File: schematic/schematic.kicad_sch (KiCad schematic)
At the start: 7 parts, among them K1 TIANBO-HJR-4102-L, U1 Pico

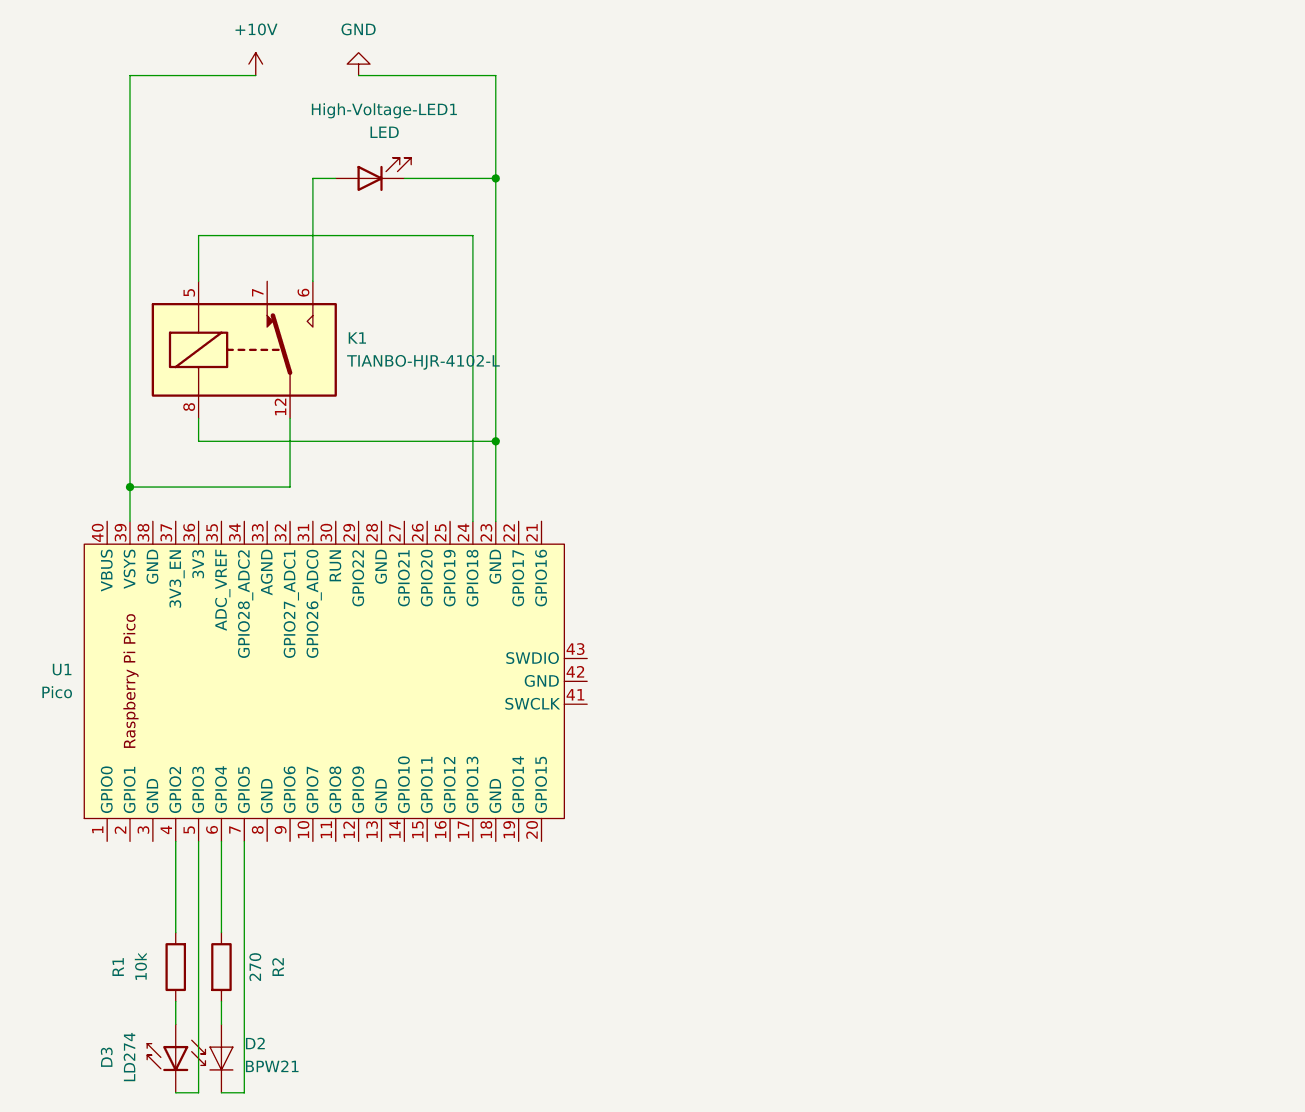
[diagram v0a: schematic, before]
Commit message: wip
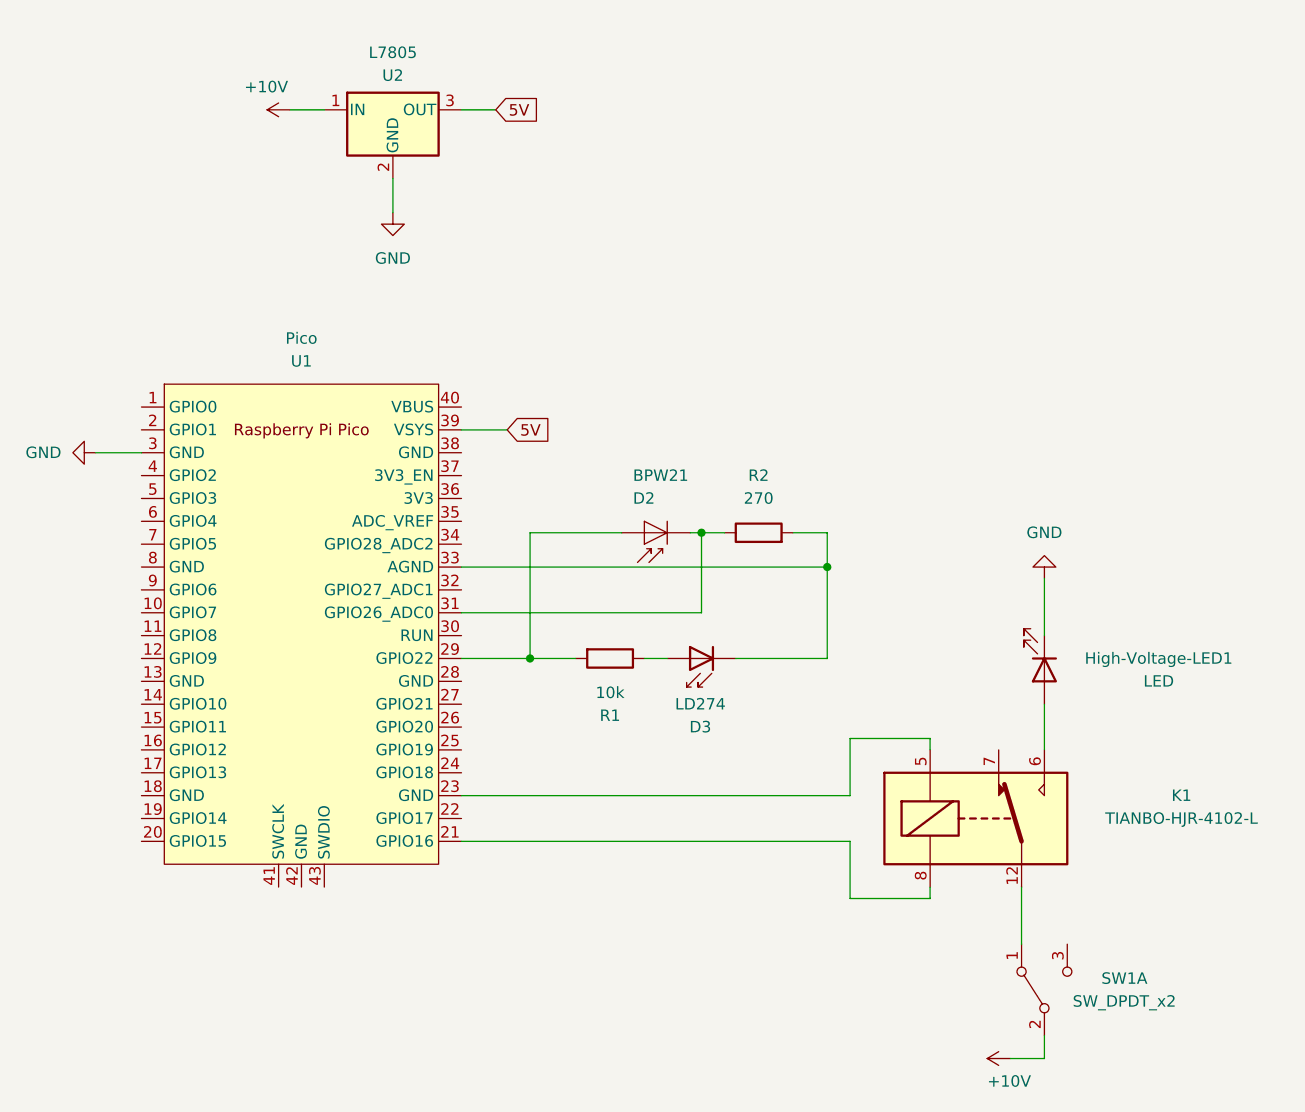
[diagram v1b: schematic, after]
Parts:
- added SW1: SW_DPDT_x2, symbol Switch:SW_DPDT_x2
- added U2: L7805, symbol Regulator_Linear:L7805
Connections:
- net +10V: now also SW1.2 (B), U2.1 (IN); no longer K1.12, U1.39 (VSYS)
- net GND: now also U1.3 (GND), U2.2 (GND); no longer K1.8, U1.23 (GND)
- net at D3.1 (K): now also R2.2, U1.33 (AGND); no longer U1.5 (GPIO3)
- net at K1.5: now also U1.23 (GND); no longer U1.24 (GPIO18)
- net at R1.2: now also D2.1 (A), U1.29 (GPIO22); no longer U1.4 (GPIO2)
- net at U1.21 (GPIO16): now also K1.8
- net at U1.31 (GPIO26_ADC0): now also D2.2 (K), R2.1
- net at U1.6 (GPIO4): no longer R2.1
- net at U1.7 (GPIO5): no longer D2.2 (K)
- new net: K1.12, SW1.1 (A)
- new net 5V: U1.39 (VSYS), U2.3 (OUT)
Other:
- moved on the sheet: D2, D3, High-Voltage-LED1, K1, R1, R2, U1
